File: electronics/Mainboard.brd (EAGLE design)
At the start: 310 x 150 mm, 225 parts, among them J1 JST_PH_B3B-PH-K-S(LF)(SN), J10 JST_PH_B3B-PH-K-S(LF)(SN), J11 JST_PH_B3B-PH-K-S(LF)(SN), J12 JST_PH_B3B-PH-K-S(LF)(SN), J13 JST_PH_B3B-PH-K-S(LF)(SN), J14 JST_PH_B3B-PH-K-S(LF)(SN), J15 JST_PH_B3B-PH-K-S(LF)(SN), J16 JST_PH_B3B-PH-K-S(LF)(SN), J17 JST_PH_B3B-PH-K-S(LF)(SN), J18 JST_PH_B3B-PH-K-S(LF)(SN), J19 JST_PH_B3B-PH-K-S(LF)(SN), J2 JST_PH_B3B-PH-K-S(LF)(SN), J20 JST_PH_B3B-PH-K-S(LF)(SN), J21 JST_PH_B3B-PH-K-S(LF)(SN), J22 JST_PH_B3B-PH-K-S(LF)(SN), J23 JST_PH_B3B-PH-K-S(LF)(SN), J24 JST_PH_B3B-PH-K-S(LF)(SN), J25 JST_PH_B3B-PH-K-S(LF)(SN), J26 JST_PH_B3B-PH-K-S(LF)(SN), J27 JST_PH_B3B-PH-K-S(LF)(SN), J28 JST_PH_B3B-PH-K-S(LF)(SN), J29 JST_PH_B3B-PH-K-S(LF)(SN), J3 JST_PH_B3B-PH-K-S(LF)(SN), J30 JST_PH_B3B-PH-K-S(LF)(SN), J31 JST_PH_B3B-PH-K-S(LF)(SN), J32 JST_PH_B3B-PH-K-S(LF)(SN), J4 JST_PH_B3B-PH-K-S(LF)(SN), J5 JST_PH_B3B-PH-K-S(LF)(SN), J6 JST_PH_B3B-PH-K-S(LF)(SN), J7 JST_PH_B3B-PH-K-S(LF)(SN), J8 JST_PH_B3B-PH-K-S(LF)(SN), J9 JST_PH_B3B-PH-K-S(LF)(SN), U15 AD5360BSTZ, U16 ADR425ARZ, U18 AD7730BRUZ, U19 AD5360BSTZ, U20 ADR425ARZ, U21 AD7730BRUZ, U22 STM32F103RCT6, U23 AD7730BRUZ, U24 AD7730BRUZ, U25 AD7730BRUZ, U26 AD7730BRUZ, U27 AD7730BRUZ, U28 AD7730BRUZ, U38 AD7730BRUZ, U39 AD7730BRUZ, U4 ADR421ARZ, U40 STM32F103RCT6, U41 AD7730BRUZ, U42 AD7730BRUZ, U43 AD7730BRUZ, U44 AD7730BRUZ, U45 AD7730BRUZ, U46 AD7730BRUZ, U5 AD7616BSTZ, U6 74AHC1G04GW/T1, U7 ADR421ARZ, U8 AD7616BSTZ, U9 74AHC1G04GW/T1, X1 22-23-2031, Y3 KC2520B-C1, Y4 ABM3B, Y7 KC2520B-C1, Y8 ABM3B

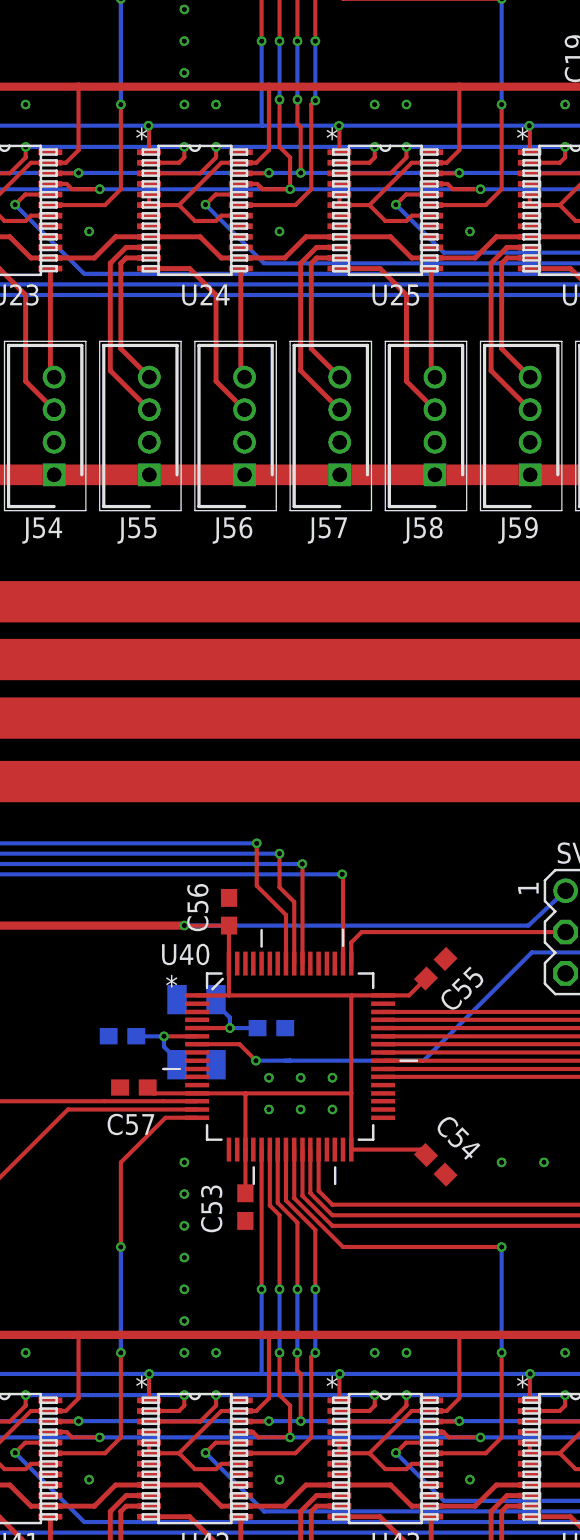
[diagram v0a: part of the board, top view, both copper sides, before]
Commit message: minor changes on names and routing
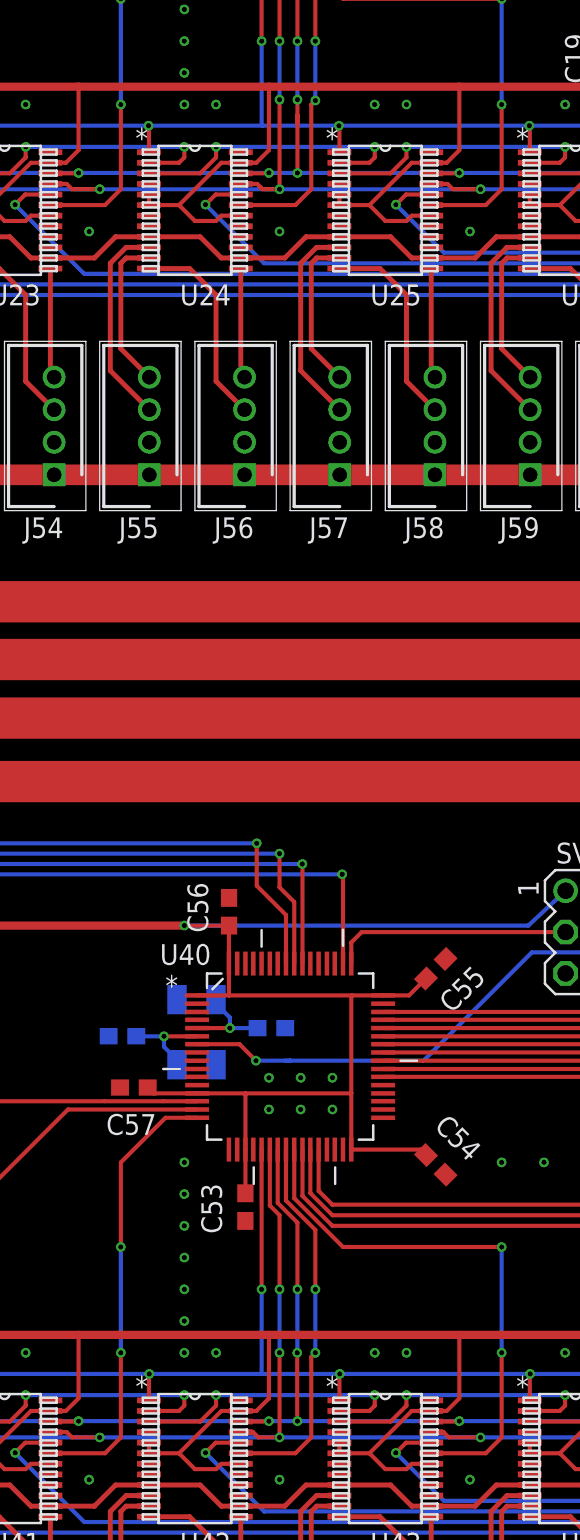
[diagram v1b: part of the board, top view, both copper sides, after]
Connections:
- net N$1 renamed RPI_PWR
- net N$41 renamed ADC_2_CONVST
- net N$77 renamed ADC_1_CONVST
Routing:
- net LC_1_SPI1_MISO: track 125.6 -> 124.7 mm
- net LC_2_SPI1_MISO: track 125.4 -> 124.5 mm
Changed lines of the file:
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@@
 <contactref element="U27" pad="21"/>
 <contactref element="U28" pad="21"/>
-<wire x1="213.2" y1="100.75" x2="224.9" y2="100.75" width="0.254" layer="16"/>
-<wire x1="224.9" y1="100.75" x2="236.6" y2="100.75" width="0.254" layer="16"/>
-<via x="224.9" y="100.75" extent="1-16" drill="0.3048"/>
+<wire x1="213.2" y1="100.75" x2="224.25" y2="100.75" width="0.254" layer="16"/>
+<wire x1="224.25" y1="100.75" x2="236.6" y2="100.75" width="0.254" layer="16"/>
+<via x="224.25" y="100.75" extent="1-16" drill="0.3048"/>
 <wire x1="236.6" y1="100.75" x2="248.3" y2="100.75" width="0.254" layer="16"/>
 <wire x1="248.3" y1="100.75" x2="260" y2="100.75" width="0.254" layer="16"/>
@@
 <wire x1="223.075" y1="100.875" x2="223.2" y2="100.75" width="0.254" layer="1"/>
 <wire x1="223.075" y1="100.875" x2="223.2" y2="100.75" width="0.254" layer="1"/>
-<wire x1="223.2" y1="100.75" x2="224.9" y2="100.75" width="0.254" layer="1"/>
+<wire x1="223.2" y1="100.75" x2="224.25" y2="100.75" width="0.254" layer="1"/>
 <wire x1="233.5694" y1="101.074996875" x2="234.575003125" y2="101.074996875" width="0.254" layer="1"/>
 <wire x1="234.575003125" y1="101.074996875" x2="234.9" y2="100.75" width="0.254" layer="1"/>
@@
 <wire x1="224.25" y1="109.85" x2="224.25" y2="106.25" width="0.254" layer="16"/>
 <via x="224.25" y="106.25" extent="1-16" drill="0.3048"/>
-<wire x1="224.9" y1="102.7" x2="224.9" y2="100.75" width="0.254" layer="1"/>
-<wire x1="224.25" y1="103.35" x2="224.9" y2="102.7" width="0.254" layer="1"/>
-<wire x1="224.25" y1="106.25" x2="224.25" y2="103.35" width="0.254" layer="1"/>
+<wire x1="224.25" y1="106.25" x2="224.25" y2="100.75" width="0.254" layer="1"/>
 </signal>
 <signal name="LC_1_SPI1_MOSI">
@@
 <wire x1="211.9" y1="101.75" x2="216.45" y2="101.75" width="0.254" layer="16"/>
 <wire x1="216.45" y1="101.75" x2="223.6" y2="101.75" width="0.254" layer="16"/>
-<wire x1="223.6" y1="101.75" x2="225.55" y2="101.75" width="0.254" layer="16"/>
-<wire x1="225.55" y1="101.75" x2="235.3" y2="101.75" width="0.254" layer="16"/>
+<wire x1="223.6" y1="101.75" x2="225.35" y2="101.75" width="0.254" layer="16"/>
+<wire x1="225.35" y1="101.75" x2="235.3" y2="101.75" width="0.254" layer="16"/>
 <wire x1="235.3" y1="101.75" x2="247" y2="101.75" width="0.254" layer="16"/>
 <wire x1="247" y1="101.75" x2="258.7" y2="101.75" width="0.254" layer="16"/>
@@
 <via x="225.35" y="109.85" extent="1-16" drill="0.3048"/>
 <via x="225.35" y="106.25" extent="1-16" drill="0.3048"/>
-<via x="225.55" y="101.75" extent="1-16" drill="0.3048"/>
+<via x="225.35" y="101.75" extent="1-16" drill="0.3048"/>
 <wire x1="224.138" y1="115.162" x2="225.35" y2="113.95" width="0.254" layer="1"/>
-<wire x1="225.55" y1="104.5747375" x2="225.55" y2="101.75" width="0.254" layer="1"/>
-<wire x1="225.35" y1="106.25" x2="225.35" y2="104.7747375" width="0.254" layer="1"/>
-<wire x1="225.35" y1="104.7747375" x2="225.55" y2="104.5747375" width="0.254" layer="1"/>
+<wire x1="225.35" y1="106.25" x2="225.35" y2="105.3" width="0.254" layer="1"/>
+<wire x1="225.35" y1="105.3" x2="225.35" y2="104.7747375" width="0.254" layer="1"/>
 <wire x1="225.35" y1="109.85" x2="225.35" y2="106.25" width="0.254" layer="16"/>
+<wire x1="225.35" y1="101.75" x2="225.35" y2="105.3" width="0.254" layer="1"/>
 </signal>
 <signal name="BT_1_MCLK_OUT">
@@
 <contactref element="U45" pad="21"/>
 <contactref element="U46" pad="21"/>
-<wire x1="213.2" y1="24.05" x2="224.9" y2="24.05" width="0.254" layer="16"/>
-<wire x1="224.9" y1="24.05" x2="236.6" y2="24.05" width="0.254" layer="16"/>
+<wire x1="213.2" y1="24.05" x2="224.25" y2="24.05" width="0.254" layer="16"/>
+<wire x1="224.25" y1="24.05" x2="236.6" y2="24.05" width="0.254" layer="16"/>
 <wire x1="236.6" y1="24.05" x2="248.3" y2="24.05" width="0.254" layer="16"/>
 <wire x1="248.3" y1="24.05" x2="260" y2="24.05" width="0.254" layer="16"/>
@@
 <wire x1="221.8694" y1="24.374996875" x2="222.625003125" y2="24.374996875" width="0.254" layer="1"/>
 <wire x1="222.625003125" y1="24.374996875" x2="222.95" y2="24.05" width="0.254" layer="1"/>
-<wire x1="222.95" y1="24.05" x2="224.9" y2="24.05" width="0.254" layer="1"/>
-<via x="224.9" y="24.05" extent="1-16" drill="0.3048"/>
+<wire x1="222.95" y1="24.05" x2="224.25" y2="24.05" width="0.254" layer="1"/>
+<via x="224.25" y="24.05" extent="1-16" drill="0.3048"/>
 <wire x1="233.5694" y1="24.374996875" x2="234.325003125" y2="24.374996875" width="0.254" layer="1"/>
 <wire x1="234.325003125" y1="24.374996875" x2="234.65" y2="24.05" width="0.254" layer="1"/>
@@
 <wire x1="224.25" y1="33.15" x2="224.25" y2="29.25" width="0.254" layer="16"/>
 <via x="224.25" y="29.25" extent="1-16" drill="0.3048"/>
-<wire x1="224.25" y1="29.25" x2="224.25" y2="26.65" width="0.254" layer="1"/>
-<wire x1="224.25" y1="26.65" x2="224.9" y2="26" width="0.254" layer="1"/>
-<wire x1="224.9" y1="26" x2="224.9" y2="24.05" width="0.254" layer="1"/>
+<wire x1="224.25" y1="29.25" x2="224.25" y2="24.05" width="0.254" layer="1"/>
 </signal>
 <signal name="LC_2_SPI1_MOSI">
@@
 <wire x1="211.9" y1="25.05" x2="216.45" y2="25.05" width="0.254" layer="16"/>
 <wire x1="216.45" y1="25.05" x2="223.6" y2="25.05" width="0.254" layer="16"/>
-<wire x1="223.6" y1="25.05" x2="225.55" y2="25.05" width="0.254" layer="16"/>
-<wire x1="225.55" y1="25.05" x2="228.15" y2="25.05" width="0.254" layer="16"/>
+<wire x1="223.6" y1="25.05" x2="225.35" y2="25.05" width="0.254" layer="16"/>
+<wire x1="225.35" y1="25.05" x2="228.15" y2="25.05" width="0.254" layer="16"/>
 <wire x1="228.15" y1="25.05" x2="235.3" y2="25.05" width="0.254" layer="16"/>
 <wire x1="235.3" y1="25.05" x2="247" y2="25.05" width="0.254" layer="16"/>
@@
 <wire x1="225.35" y1="29.2636" x2="225.3364" y2="29.25" width="0.254" layer="16"/>
 <via x="225.3364" y="29.25" extent="1-16" drill="0.3048"/>
-<via x="225.55" y="25.05" extent="1-16" drill="0.3048"/>
-<wire x1="225.3364" y1="29.25" x2="225.3364" y2="28.1636" width="0.254" layer="1"/>
-<wire x1="225.3364" y1="28.1636" x2="225.55" y2="27.95" width="0.254" layer="1"/>
-<wire x1="225.55" y1="27.95" x2="225.55" y2="25.05" width="0.254" layer="1"/>
+<via x="225.35" y="25.05" extent="1-16" drill="0.3048"/>
+<wire x1="225.3364" y1="25.0636" x2="225.35" y2="25.05" width="0.254" layer="1"/>
+<wire x1="225.3364" y1="29.25" x2="225.3364" y2="25.0636" width="0.254" layer="1"/>
 </signal>
 <signal name="BT2_1_MCLK_OUT">
@@
 <wire x1="61.1" y1="115.7" x2="64.0394" y2="118.6394" width="0.4064" layer="16"/>
 </signal>
-<signal name="N$41">
+<signal name="ADC_2_CONVST">
 <contactref element="U5" pad="68"/>
 <contactref element="U6" pad="4"/>
@@
 <wire x1="26.4" y1="105.5" x2="28" y2="105.5" width="0.4064" layer="1"/>
 </signal>
-<signal name="N$77">
+<signal name="ADC_1_CONVST">
 <contactref element="U8" pad="68"/>
 <contactref element="U9" pad="4"/>
@@
 <wire x1="291.85" y1="120.28" x2="291.85" y2="97.8" width="0.4064" layer="1"/>
 </signal>
-<signal name="N$1">
+<signal name="RPI_PWR">
 <contactref element="SV1" pad="4"/>
 <contactref element="SV1" pad="2"/>
